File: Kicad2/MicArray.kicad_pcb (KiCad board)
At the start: 2 copper layers, 176.6 x 176.6 mm, 68 parts, among them J1 Conn_01x06, U1 AP2204RB-3.3

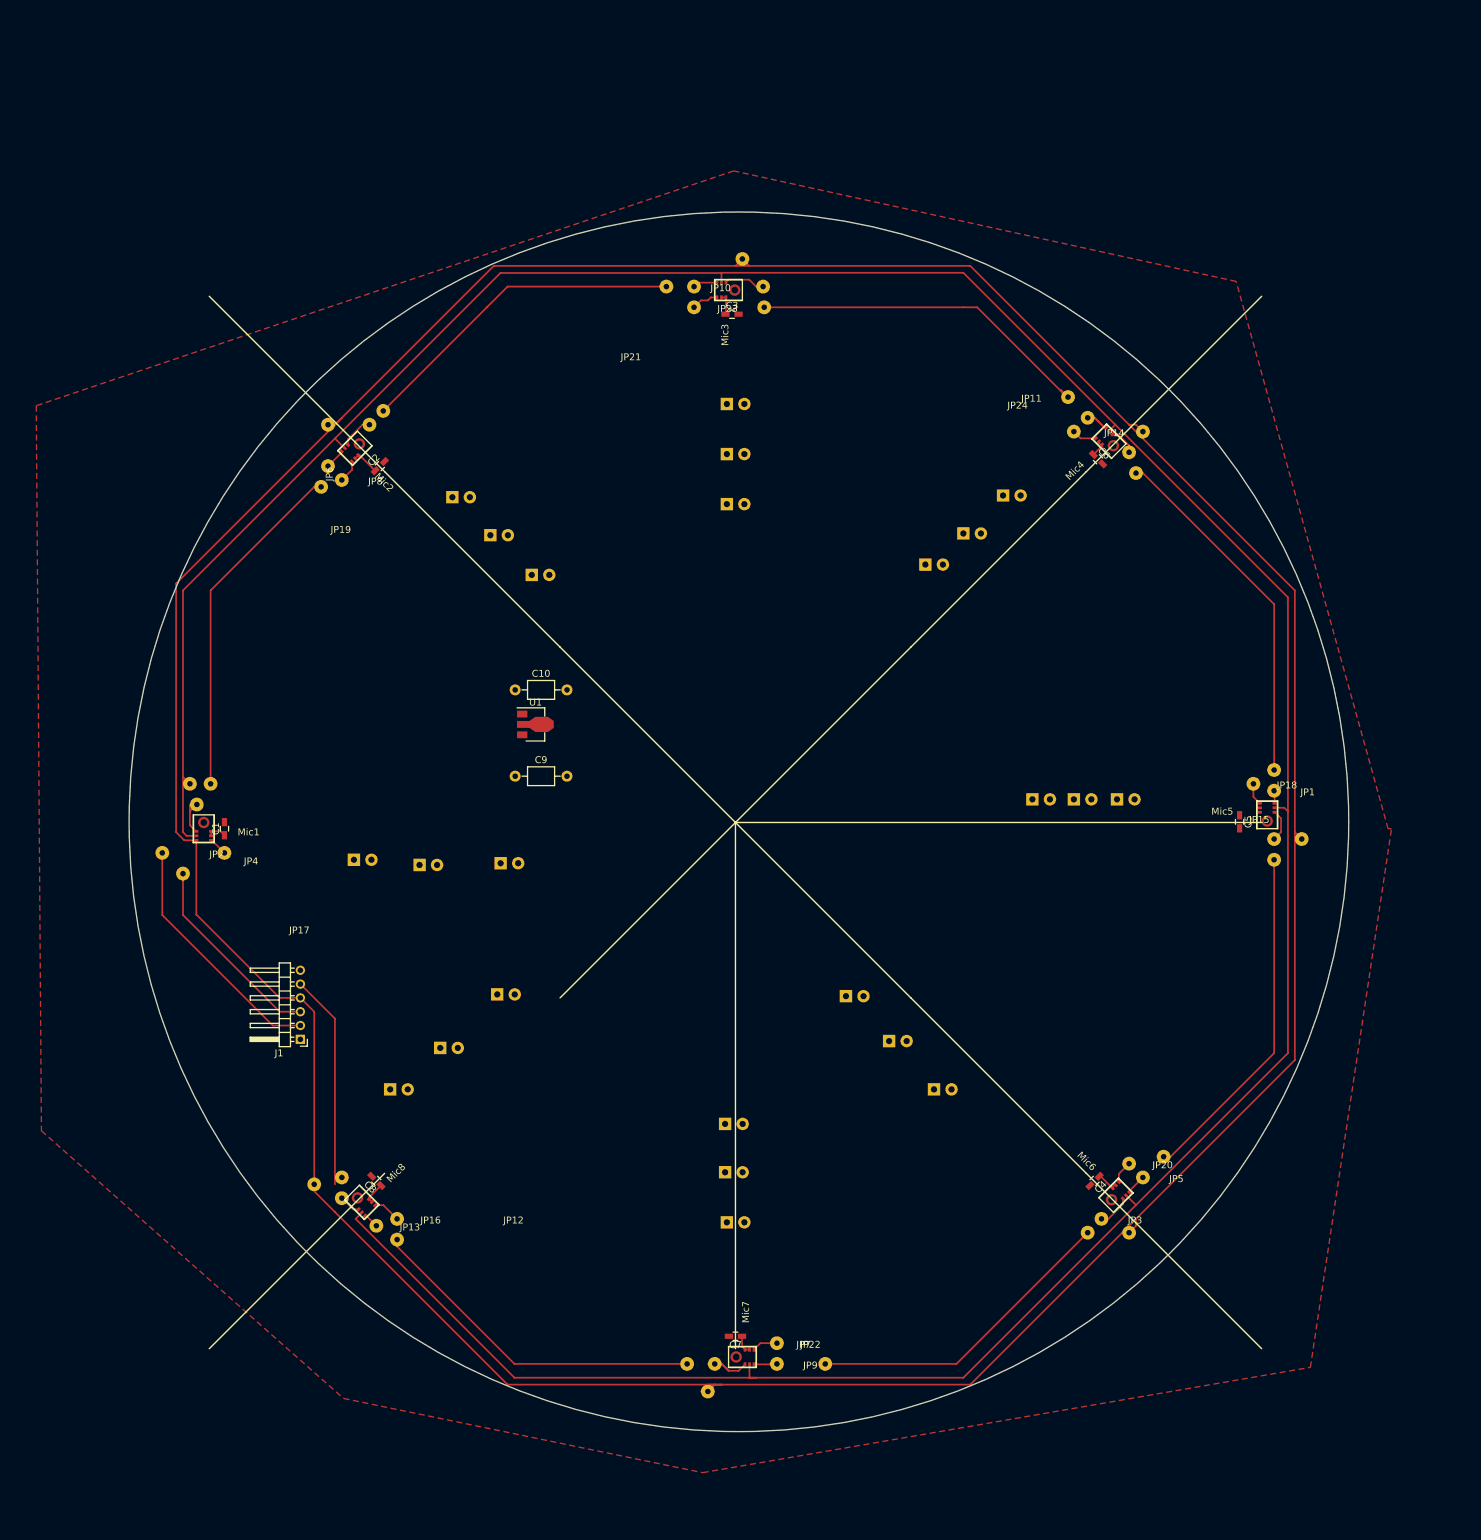
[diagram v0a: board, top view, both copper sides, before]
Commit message: Add files via upload
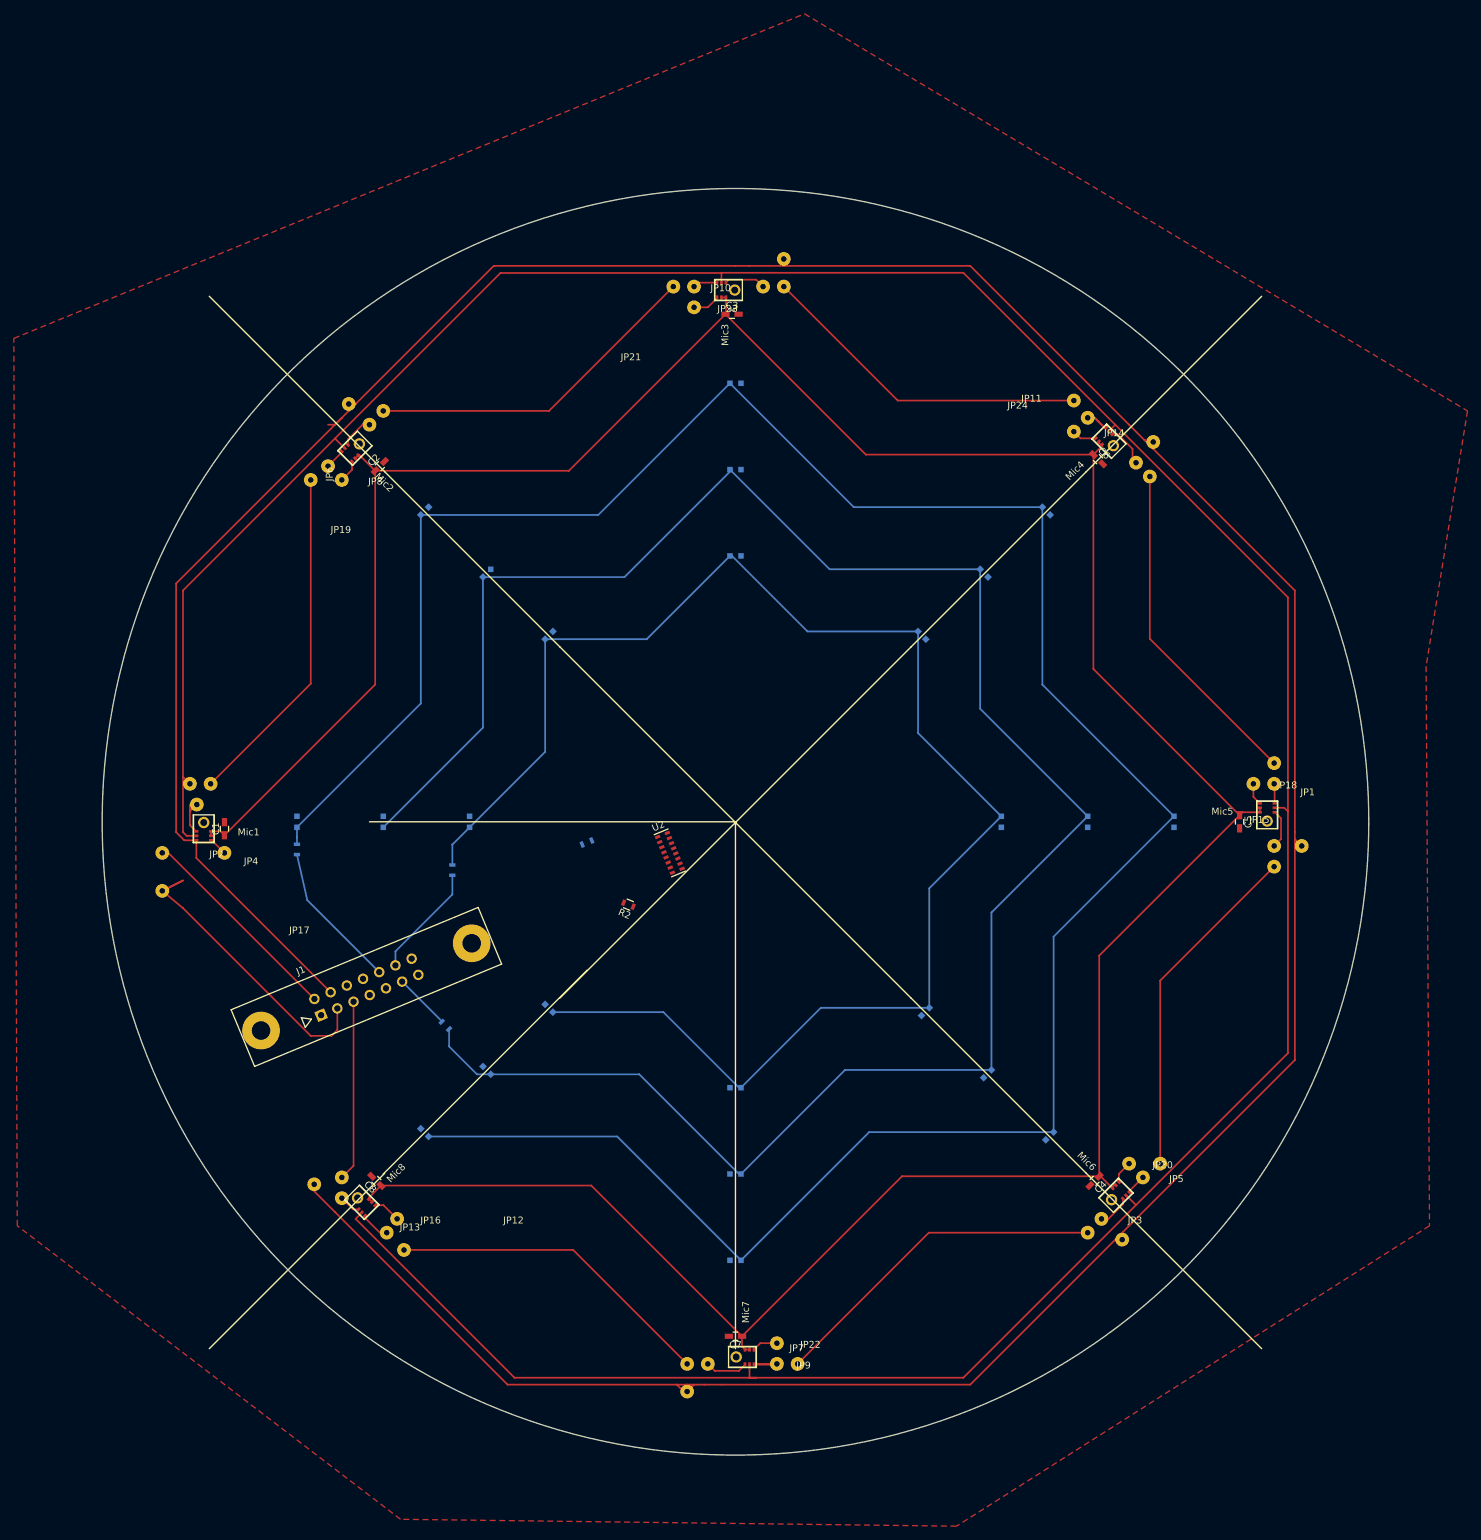
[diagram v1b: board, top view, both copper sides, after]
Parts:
- removed C10, C9: C, Capacitors_THT:C_Axial_L3.8mm_D2.6mm_P7.50mm_Horizontal
- removed U1: AP2204RB-3.3, TO_SOT_Packages_SMD:SOT-89-3
- added R1: 1k, Resistors_SMD:R_0603, B.Cu at (105.5, 104.5)
- added R11: 220, Resistors_SMD:R_0603, B.Cu at (86.0, 108.5)
- added R2: 1k, Resistors_SMD:R_0603, F.Cu at (111.5, 113.5)
- added R3: 220, Resistors_SMD:R_0603, B.Cu at (63.5, 105.5)
- added R9: 220, Resistors_SMD:R_0603, B.Cu at (85.0, 131.0)
- added U2: SN74HC138, Resistors_SMD:R_Cat16-8, F.Cu at (117.5, 106.0)
- D1, D10, D11, D12, D13, D14, D15, D16, D17, D18, D19, D2, D20, D21, D22, D23, D24, D3, D4, D5, D6, D7, D8, D9: footprint LEDs:LED_D1.8mm_W1.8mm_H2.4mm_Horizontal_O1.27mm_Z1.6mm -> LEDs:LED_0603
- J1: value Conn_01x06 -> Conn_01x12_Male; footprint Pin_Headers:Pin_Header_Angled_1x06_Pitch2.00mm -> Connectors:he10-14d
- moved D21 93.9 mm to (165.5, 101.5), turned to 90 degrees
- moved D9 82.8 mm to (88.5, 101.5), turned to 270 degrees
- moved D1 81.9 mm to (63.5, 101.5), turned to 270 degrees
- moved D10 79.6 mm to (100.0, 74.5), turned to 225 degrees
- moved D5 78.3 mm to (76.0, 101.5), turned to 270 degrees
- moved D22 76.3 mm to (154.5, 129.0), turned to 45 degrees
- moved D4 75.1 mm to (172.0, 56.5), turned to 135 degrees
- moved D17 73.0 mm to (178.0, 101.5), turned to 90 degrees
- moved D11 55.6 mm to (127.0, 63.0), turned to 180 degrees
- moved D13 52.1 mm to (190.5, 101.5), turned to 90 degrees
- moved D23 47.0 mm to (127.0, 140.0)
- moved D19 46.5 mm to (127.0, 152.5)
- moved D16 43.5 mm to (82.0, 146.5), turned to 315 degrees
- moved D18 43.4 mm to (163.5, 138.0), turned to 45 degrees
- moved D3 41.8 mm to (127.0, 38.0), turned to 180 degrees
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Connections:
- D1 pad 1: GND -> /LEDArray/Row1
- D1 pad 2: Net-(D1-Pad2) -> /LEDArray/LEDSA
- D10 pad 1: GND -> /LEDArray/Row2
- D10 pad 2: Net-(D10-Pad2) -> /LEDArray/LEDSC
- D11 pad 1: GND -> /LEDArray/Row3
- D11 pad 2: Net-(D11-Pad2) -> /LEDArray/LEDSC
- D12 pad 1: GND -> /LEDArray/Row4
- D12 pad 2: Net-(D12-Pad2) -> /LEDArray/LEDSC
- D13 pad 1: GND -> /LEDArray/Row5
- D13 pad 2: Net-(D13-Pad2) -> /LEDArray/LEDSA
- D14 pad 1: GND -> /LEDArray/Row6
- D14 pad 2: Net-(D14-Pad2) -> /LEDArray/LEDSA
- D15 pad 1: GND -> /LEDArray/Row7
- D15 pad 2: Net-(D15-Pad2) -> /LEDArray/LEDSA
- D16 pad 1: GND -> /LEDArray/Row8
- D16 pad 2: Net-(D16-Pad2) -> /LEDArray/LEDSA
- D17 pad 1: GND -> /LEDArray/Row5
- D17 pad 2: Net-(D17-Pad2) -> /LEDArray/LEDSB
- D18 pad 1: GND -> /LEDArray/Row6
- D18 pad 2: Net-(D18-Pad2) -> /LEDArray/LEDSB
- D19 pad 1: GND -> /LEDArray/Row7
- D19 pad 2: Net-(D19-Pad2) -> /LEDArray/LEDSB
- D2 pad 1: GND -> /LEDArray/Row2
- D2 pad 2: Net-(D2-Pad2) -> /LEDArray/LEDSA
- D20 pad 1: GND -> /LEDArray/Row8
- D20 pad 2: Net-(D20-Pad2) -> /LEDArray/LEDSB
- D21 pad 1: GND -> /LEDArray/Row5
- D21 pad 2: Net-(D21-Pad2) -> /LEDArray/LEDSC
- D22 pad 1: GND -> /LEDArray/Row6
- D22 pad 2: Net-(D22-Pad2) -> /LEDArray/LEDSC
- D23 pad 1: GND -> /LEDArray/Row7
- D23 pad 2: Net-(D23-Pad2) -> /LEDArray/LEDSC
- D24 pad 1: GND -> /LEDArray/Row8
- D24 pad 2: Net-(D24-Pad2) -> /LEDArray/LEDSC
- D3 pad 1: GND -> /LEDArray/Row3
- D3 pad 2: Net-(D3-Pad2) -> /LEDArray/LEDSA
- D4 pad 1: GND -> /LEDArray/Row4
- D4 pad 2: Net-(D4-Pad2) -> /LEDArray/LEDSA
- D5 pad 1: GND -> /LEDArray/Row1
- D5 pad 2: Net-(D5-Pad2) -> /LEDArray/LEDSB
- D6 pad 1: GND -> /LEDArray/Row2
- D6 pad 2: Net-(D6-Pad2) -> /LEDArray/LEDSB
- D7 pad 1: GND -> /LEDArray/Row3
- D7 pad 2: Net-(D7-Pad2) -> /LEDArray/LEDSB
- D8 pad 1: GND -> /LEDArray/Row4
- D8 pad 2: Net-(D8-Pad2) -> /LEDArray/LEDSB
- D9 pad 1: GND -> /LEDArray/Row1
- D9 pad 2: Net-(D9-Pad2) -> /LEDArray/LEDSC
- J1 pad 1: Net-(C9-Pad1) -> Net-(C1-Pad1)
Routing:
- net Net-(C1-Pad1): track 22.3 -> 454.1 mm
- net /LEDArray/LEDSA: track 0.00 -> 371.7 mm
- net /LEDArray/LEDSB: track 0.00 -> 306.9 mm
- net /LEDArray/LEDSC: track 0.00 -> 229.4 mm
- net /SerialData: track 557.0 -> 530.9 mm
- net /LEDArray/ColSelectA: track 0.00 -> 21.5 mm
- net /LEDArray/ColSelectC: track 0.00 -> 16.5 mm
- net Net-(J1-Pad3): track 29.8 -> 44.1 mm
- net /LEDArray/ColSelectB: track 0.00 -> 8.21 mm
- net /WISO: track 31.1 -> 26.1 mm
- net Net-(J1-Pad2): track 35.6 -> 30.8 mm
- net Net-(JP20-Pad2): track 45.9 -> 49.9 mm
- net Net-(JP11-Pad2): track 52.4 -> 48.8 mm
- net Net-(JP9-Pad1): track 2.35 -> 5.70 mm
- net Net-(JP15-Pad1): track 51.9 -> 49.0 mm
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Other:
- board size 176.6 x 176.6 mm -> 183.4 x 183.4 mm
